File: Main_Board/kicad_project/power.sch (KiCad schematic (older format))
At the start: 32 parts, among them J5 PWR_ENTRY, J6 12V_HDR, J7 3V3_HDR, J8 5V_HDR, U5 TPS562200, U6 TPS562200

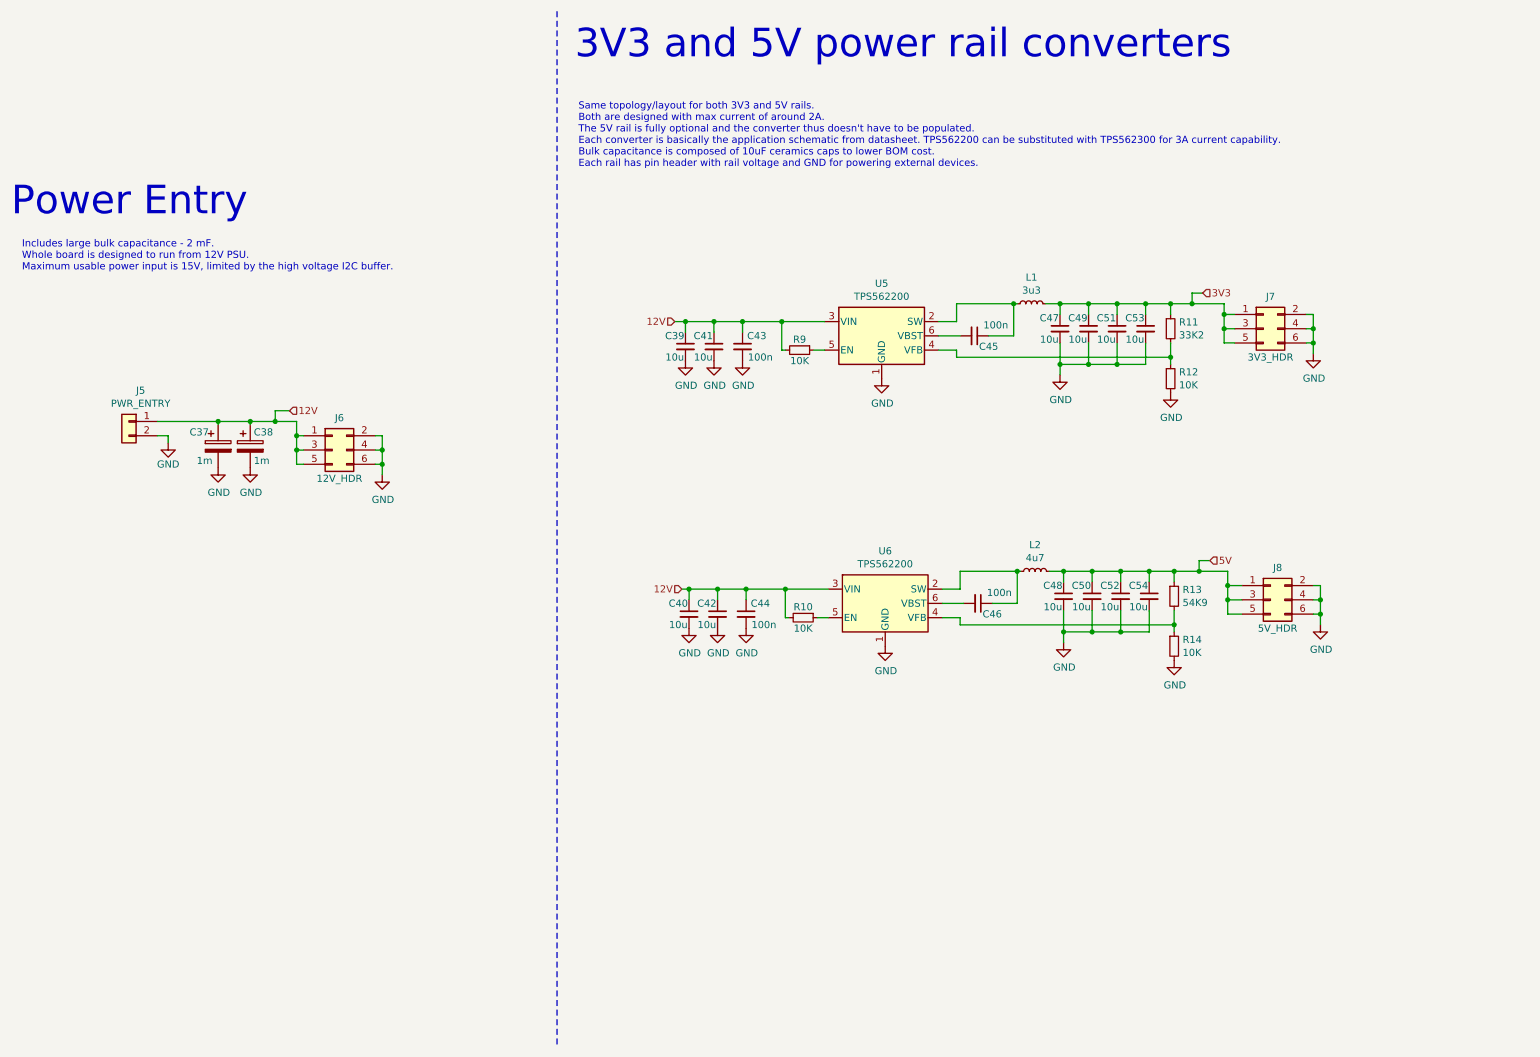
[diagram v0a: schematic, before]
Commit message: progress on MCU pinout
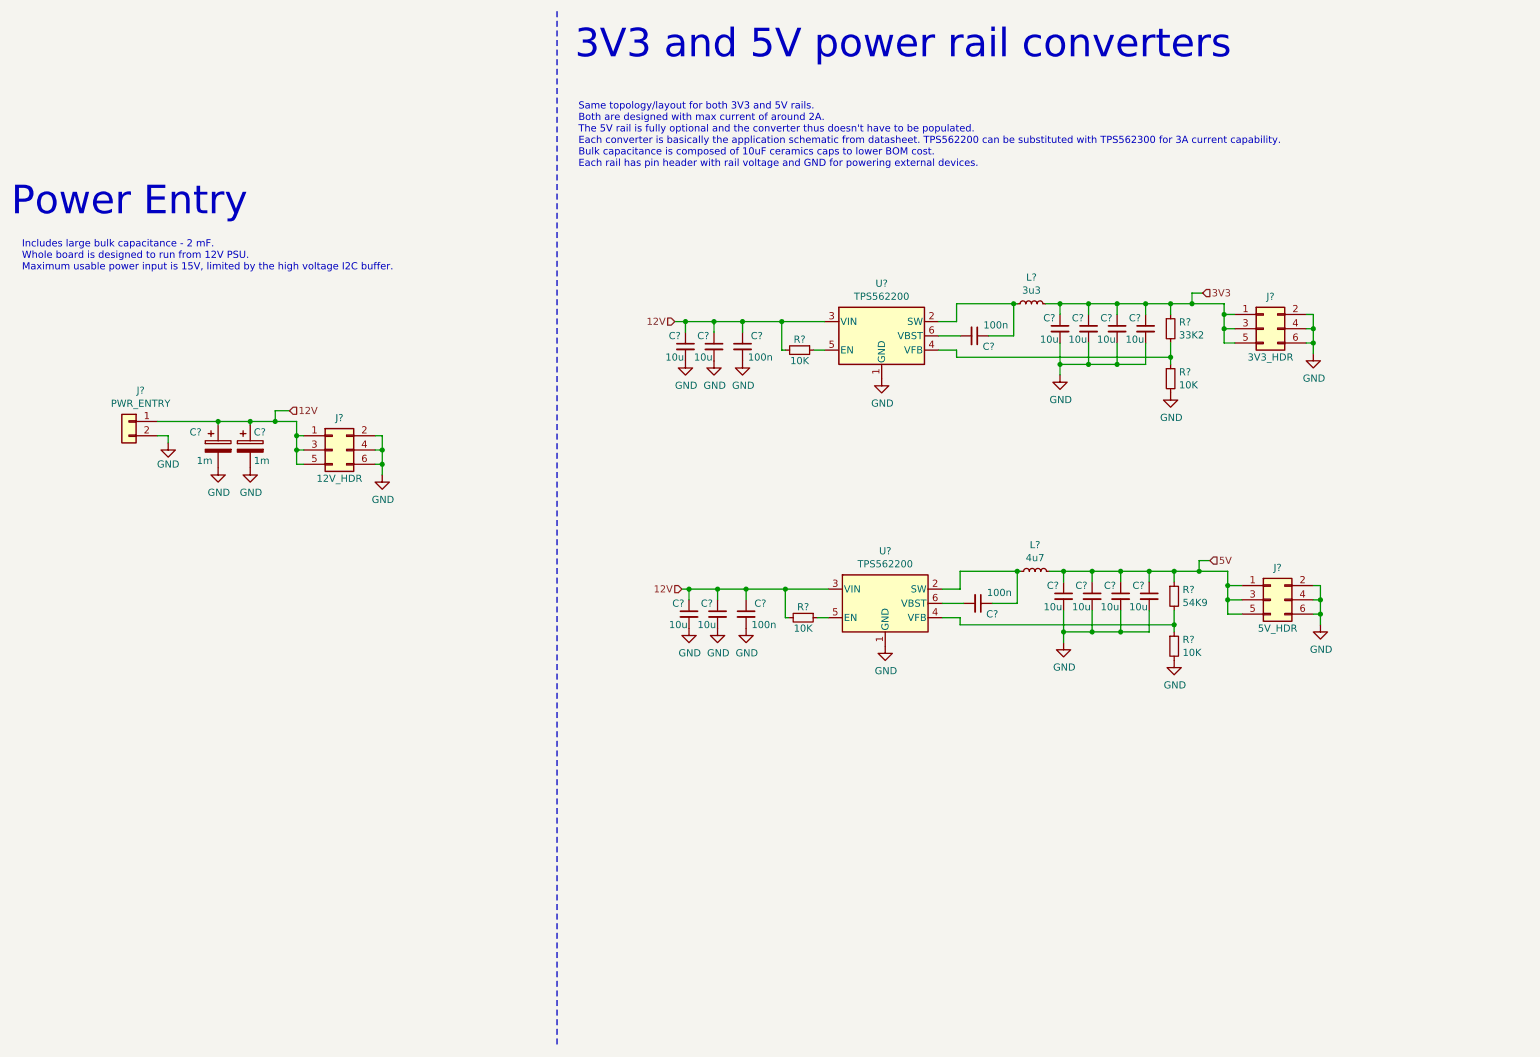
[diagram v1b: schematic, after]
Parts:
- renumbered C45 to C?, C47 to C?, C49 to C?, C51 to C?, C53 to C?, C43 to C?, C41 to C?, C39 to C?, C46 to C?, C48 to C?, C50 to C?, C52 to C?, C54 to C?, C44 to C?, C42 to C?, C40 to C?, C38 to C?, C37 to C?, J5 to J?, J7 to J?, J8 to J?, J6 to J?, L1 to L?, L2 to L?, R11 to R?, R12 to R?, R9 to R?, R13 to R?, R14 to R?, R10 to R?, U5 to U?, U6 to U?

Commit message: progress?
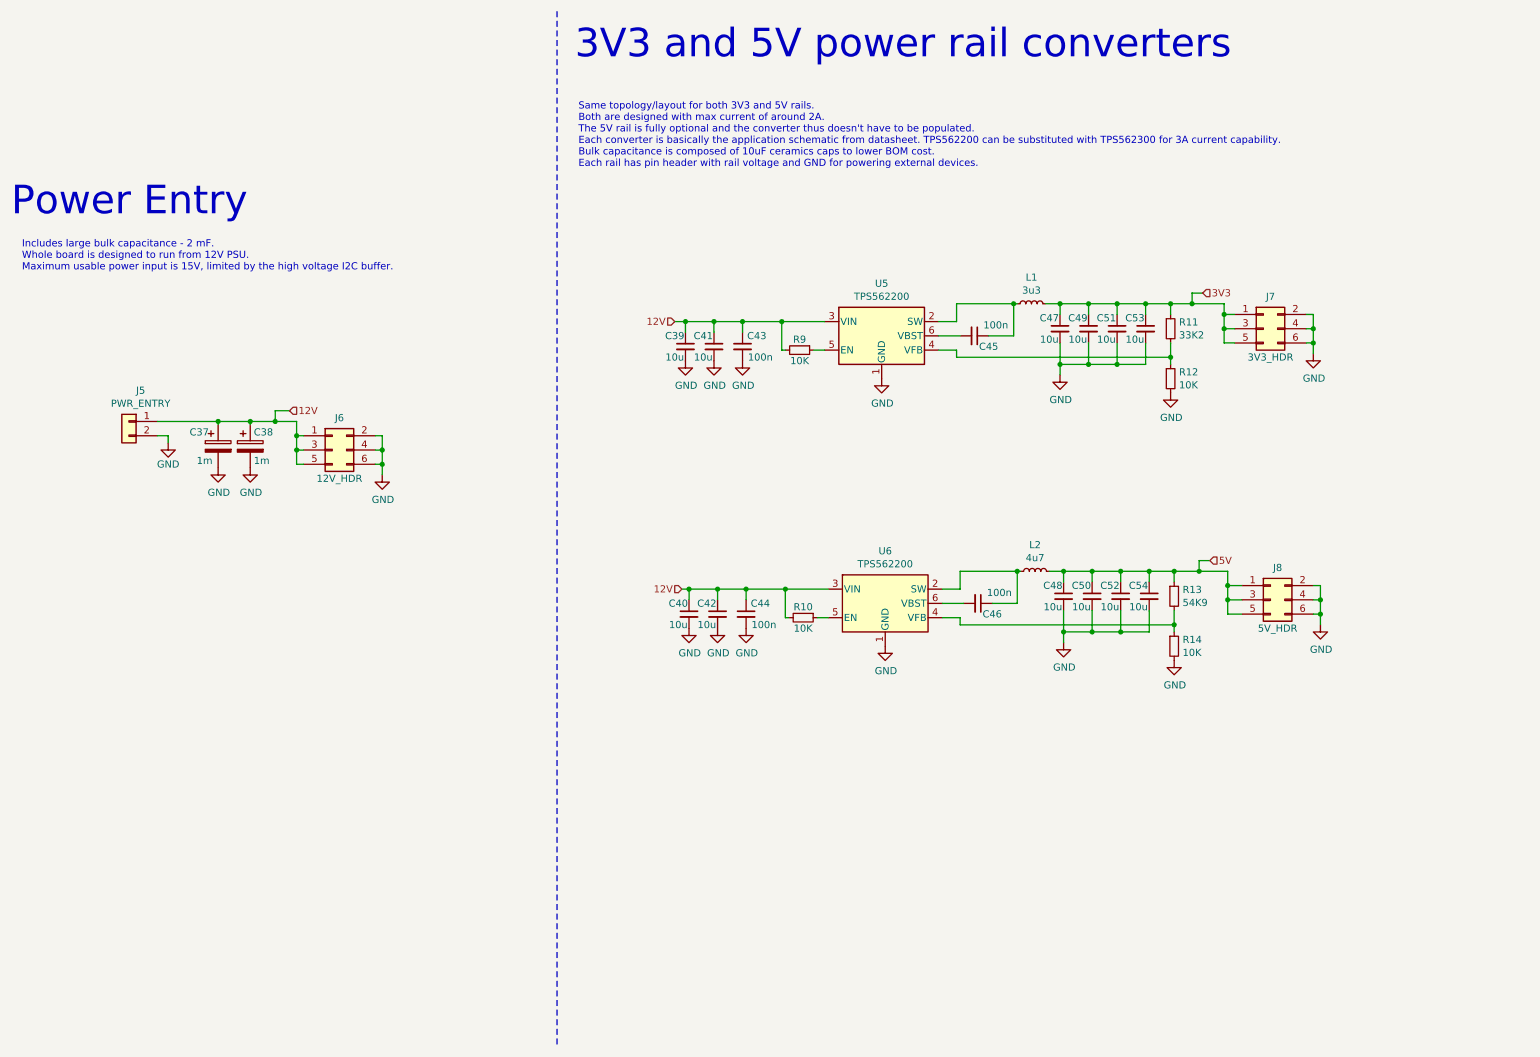
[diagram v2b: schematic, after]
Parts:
- gave numbers to parts that had none: 32
